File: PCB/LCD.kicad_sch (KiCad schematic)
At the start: 31 parts, among them J3 FH12-30S-0.5SH_55_, Q2 CSD13380F3, Q3 CSD13380F3, Q4 CSD13380F3, U1 TPS61042DRBR

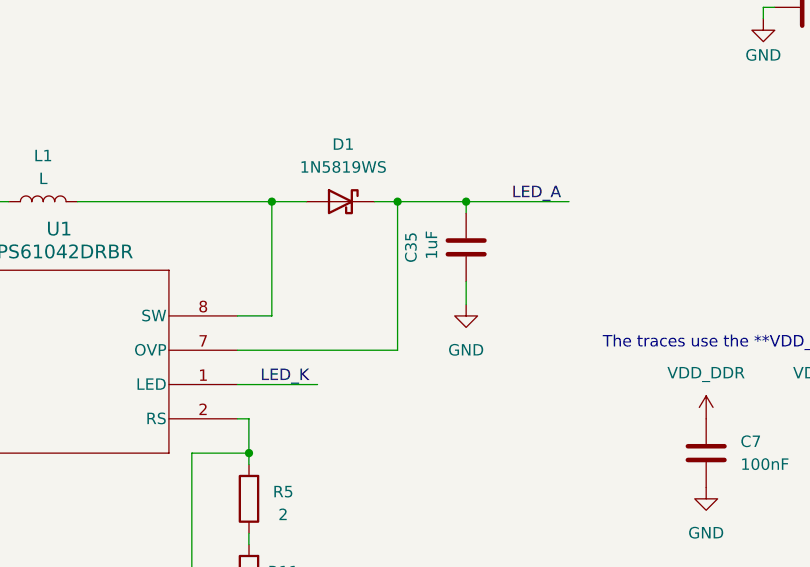
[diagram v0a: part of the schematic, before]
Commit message: pcb_update
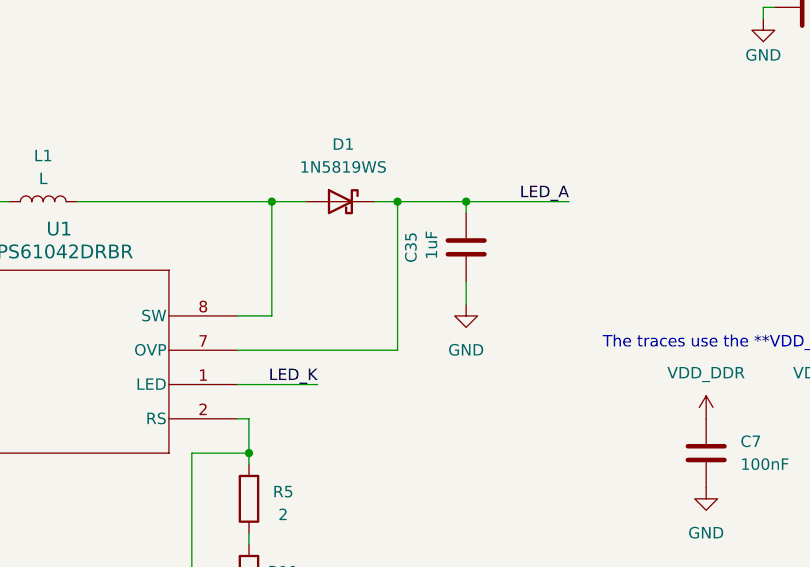
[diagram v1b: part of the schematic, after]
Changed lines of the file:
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@@
-	(wire
-		(pts
-			(xy 105.41 154.94) (xy 96.52 154.94)
-		)
-		(stroke
-			(width 0)
-			(type default)
-		)
-	)
 	(wire
 		(pts
@@
 	(wire
 		(pts
+			(xy 96.52 154.94) (xy 105.41 154.94)
+		)
+		(stroke
+			(width 0)
+			(type default)
+		)
+	)
+	(wire
+		(pts
 			(xy 254 115.57) (xy 264.16 115.57)
 		)
@@
 	)
 	(label "LED_K"
-		(at 99.06 154.94 0)
+		(at 105.41 154.94 180)
 		(effects
 			(font
 				(size 1.27 1.27)
 			)
-			(justify left bottom)
+			(justify right bottom)
 		)
 	)
 	(label "LED_A"
-		(at 127 134.62 0)
+		(at 133.35 134.62 180)
 		(effects
 			(font
 				(size 1.27 1.27)
 			)
-			(justify left bottom)
-		)
-	)
+			(justify right bottom)
+		)
+	)
